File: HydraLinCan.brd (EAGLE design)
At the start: 59.9 x 37 mm, 33 parts, among them CN1 8p-2.54, J1 HYDRABUS_SHIELD_CON_HEADER_2X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, J2 HYDRABUS_SHIELD_CON_HEADER_2X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, J3 HYDRABUS_SHIELD_CON_HEADER_2X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, K1 TS-1188E, U1 SN65HVD233DG4, U2 SN65HVD233DG4, U3 CJ78M05-to252

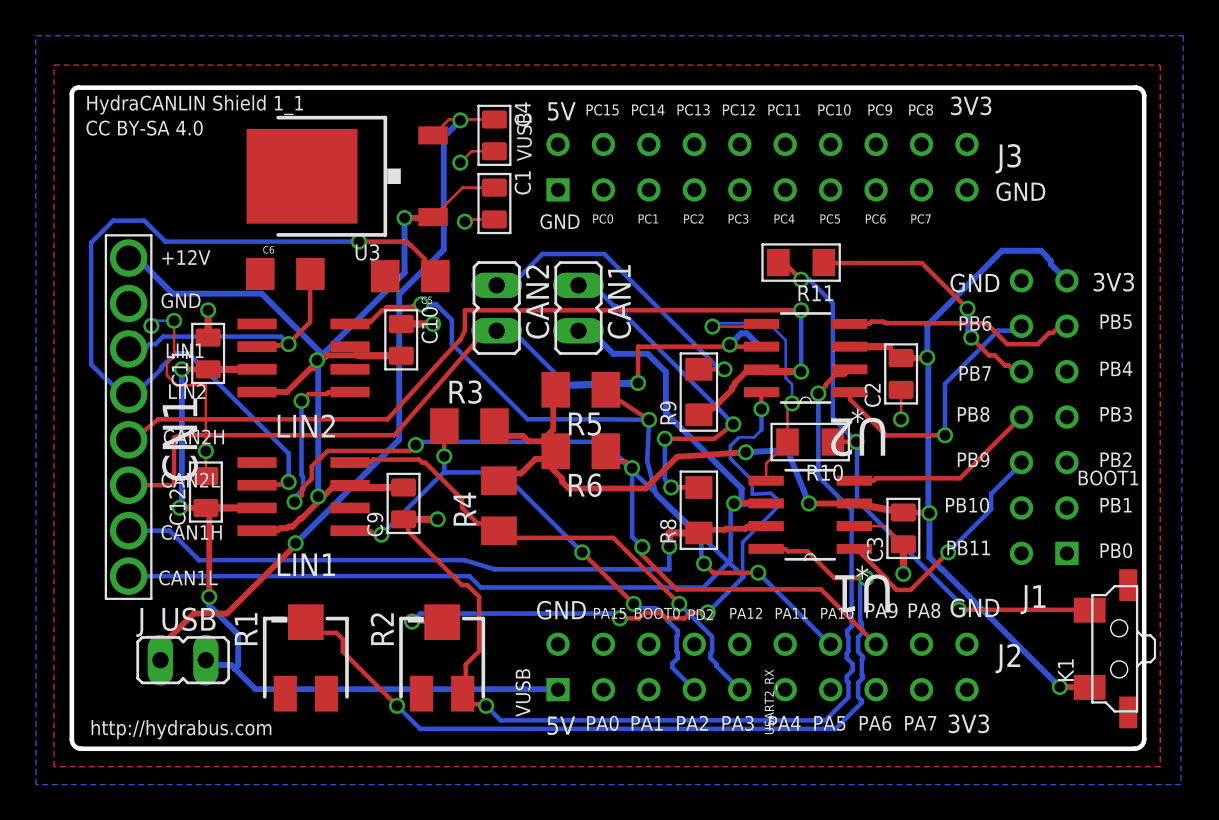
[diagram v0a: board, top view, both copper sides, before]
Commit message: 2 layers parts
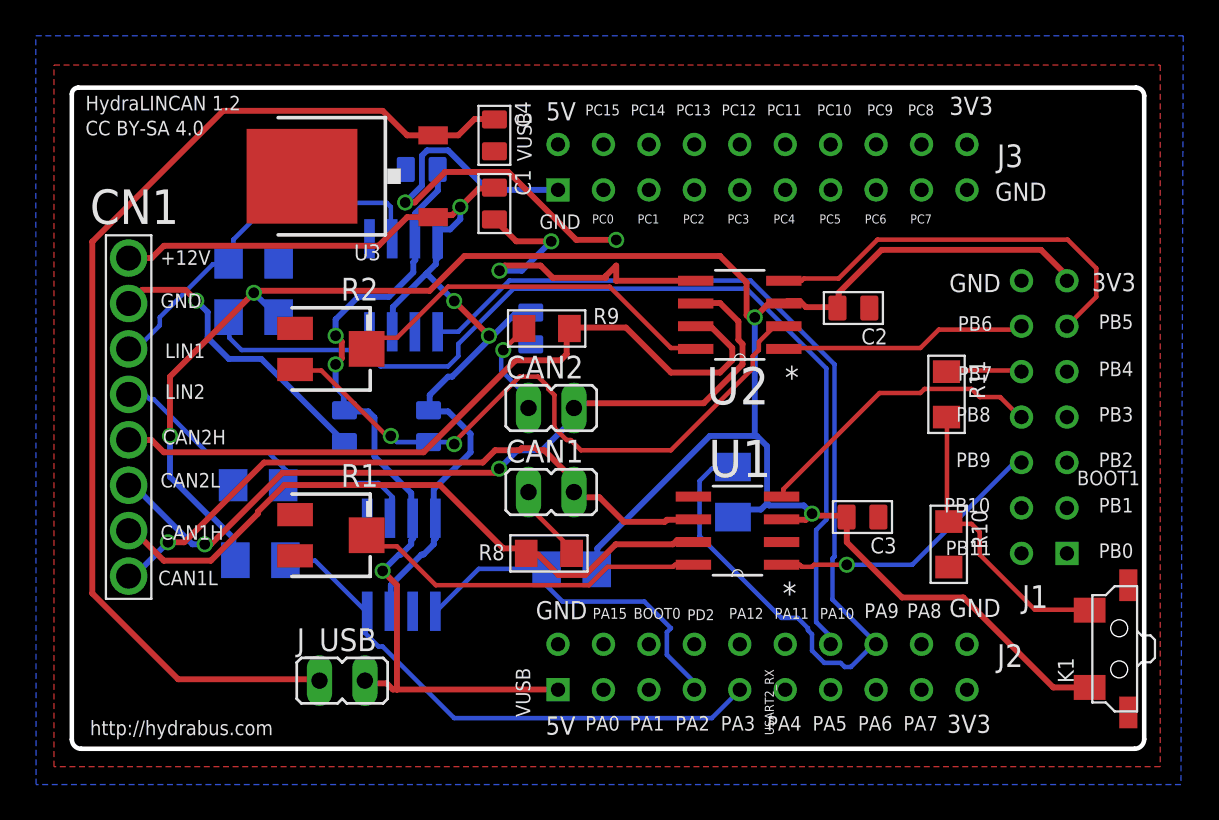
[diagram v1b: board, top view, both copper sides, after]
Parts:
- moved R5 18.7 mm to (10.2, 24.1), flipped to the bottom
- moved R2 18.4 mm to (14.5, 22.4), turned to 180 degrees
- moved C11 15.8 mm to (19.6, 32.4), flipped to the bottom, turned to 90 degrees
- moved C5 14.5 mm to (10.4, 14.7), flipped to the bottom, turned to 0 degrees
- moved R4 13.7 mm to (10.5, 10.5), flipped to the bottom, turned to 0 degrees
- moved R11 11.0 mm to (48.9, 19.8), turned to 270 degrees
- moved CAN1 10.4 mm to (26.8, 14.4), turned to 270 degrees
- moved R3 9.83 mm to (27.9, 10.0), flipped to the bottom, turned to 180 degrees
- moved R10 9.63 mm to (49.0, 11.4), turned to 270 degrees
- moved R9 9.22 mm to (26.5, 23.5), turned to 180 degrees
- moved J_USB 8.96 mm to (15.1, 3.81)
- moved R6 8.81 mm to (37.0, 14.4), flipped to the bottom, turned to 270 degrees
- moved R8 8.72 mm to (26.7, 10.9), turned to 0 degrees
- moved C12 8.58 mm to (15.2, 18.0), flipped to the bottom, turned to 0 degrees
- moved C10 7.27 mm to (25.7, 23.5), flipped to the bottom, turned to 180 degrees
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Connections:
- net N$10 renamed CAN1_P
- net N$11 renamed CAN2_N
- net N$12 renamed CAN2_P
- net N$9 renamed CAN1_N
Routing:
- net +3V3: track 77.6 -> 123.1 mm, vias 5 -> 4
- net N$1: track 48.5 -> 19.9 mm, vias 2 -> 0
- net N$4: track 46.5 -> 19.3 mm, vias 2 -> 0
- net N$17: track 47.4 -> 21.3 mm, vias 4 -> 0
- net GND: track 41.7 -> 62.3 mm, vias 11 -> 5
- net N$13: track 57.3 -> 37.1 mm, vias 3 -> 2
- net CAN1_N: track 56.9 -> 36.7 mm
- net N$15: track 42.1 -> 60.9 mm, vias 2 -> 0
- net N$21: track 32.7 -> 16.5 mm, vias 3 -> 0
- net N$19: track 20.4 -> 4.43 mm, vias 3 -> 0
- net PA10: track 41.9 -> 57.1 mm, vias 4 -> 0
- net N$16: track 17.6 -> 5.60 mm
- net PB7: track 14.4 -> 4.26 mm, vias 2 -> 0
- net PB5: track 13.1 -> 23.0 mm
- net PA2: track 30.1 -> 20.3 mm, vias 4 -> 0
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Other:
- board text added: "HydraLINCAN 1.2"
- board text removed: "HydraCANLIN Shield 1_1"
